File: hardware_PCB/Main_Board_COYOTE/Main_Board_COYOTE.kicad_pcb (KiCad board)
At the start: 2 copper layers, 73.5 x 138 mm, 47 parts, among them J1 FTDI, J2 Conn_01x05_Pin, J3 Conn_01x05_Pin, J4 V+-, J5 MOTOR_PINM1A, J6 MOTOR_PINM1B, J7 MOTOR_PINM1A, J8 MOTOR_PINM1B, Q1 2N7002, SW1 SW_SPST, SW2 START, SW3 START, U1 TA6586, U2 ESP32-WROOM-32, U3 AMS1117-3.3, U4 LM7805_TO220, U5 TA6586

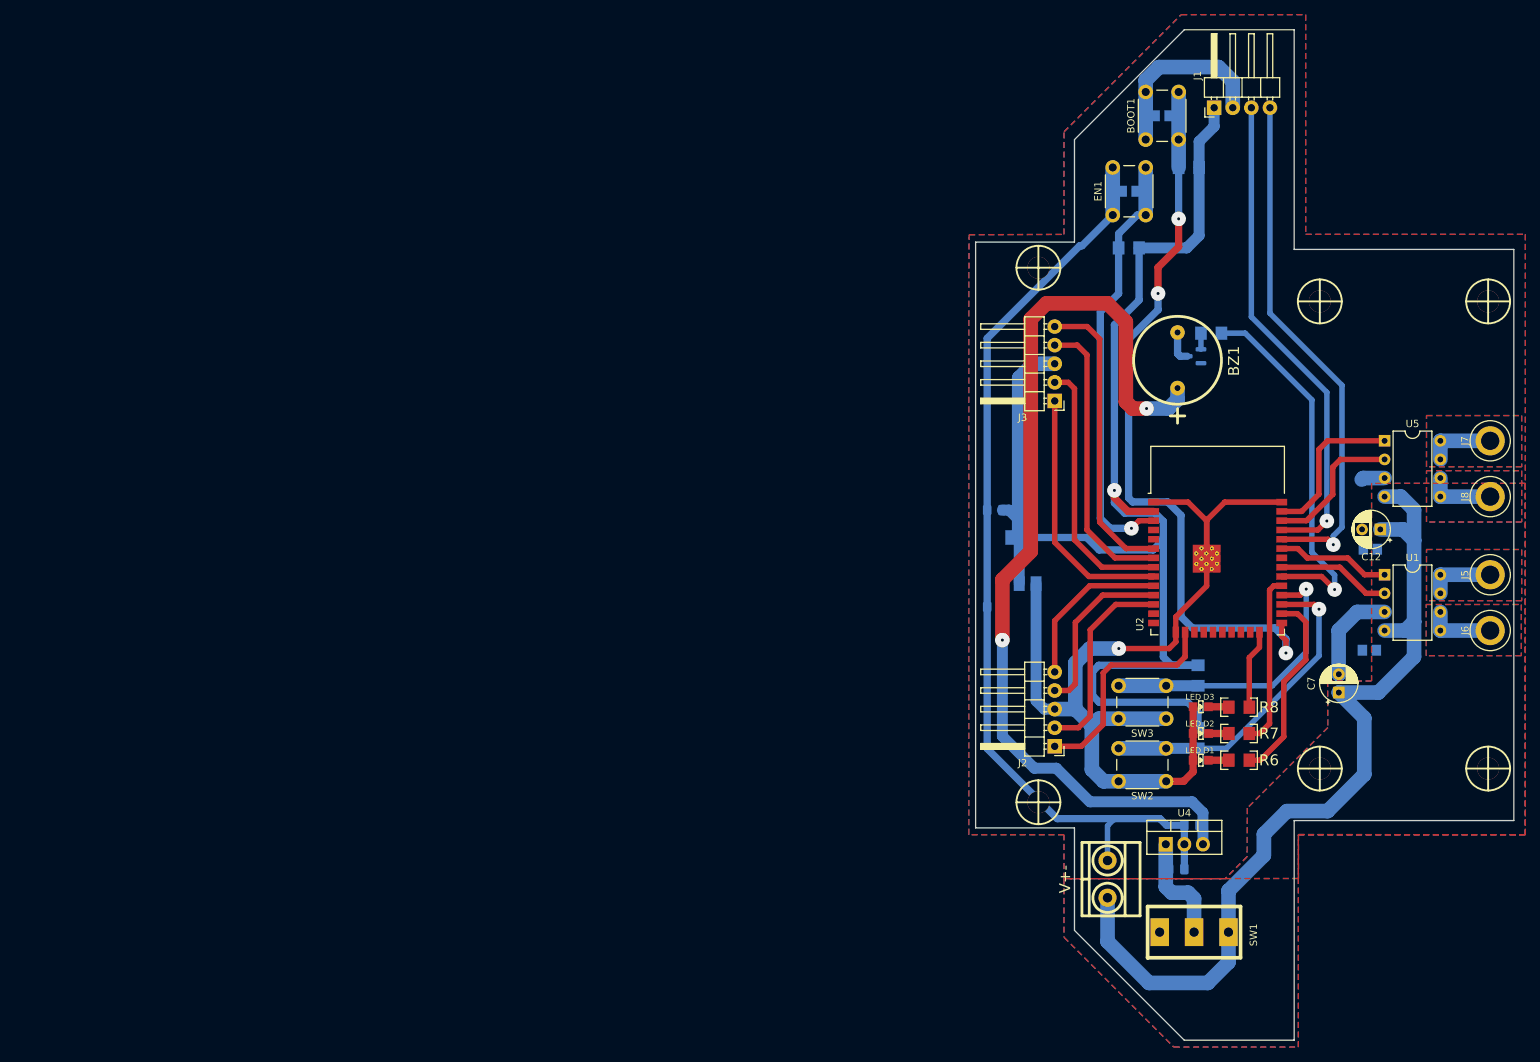
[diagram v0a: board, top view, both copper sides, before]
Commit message: Terminados los PCBs
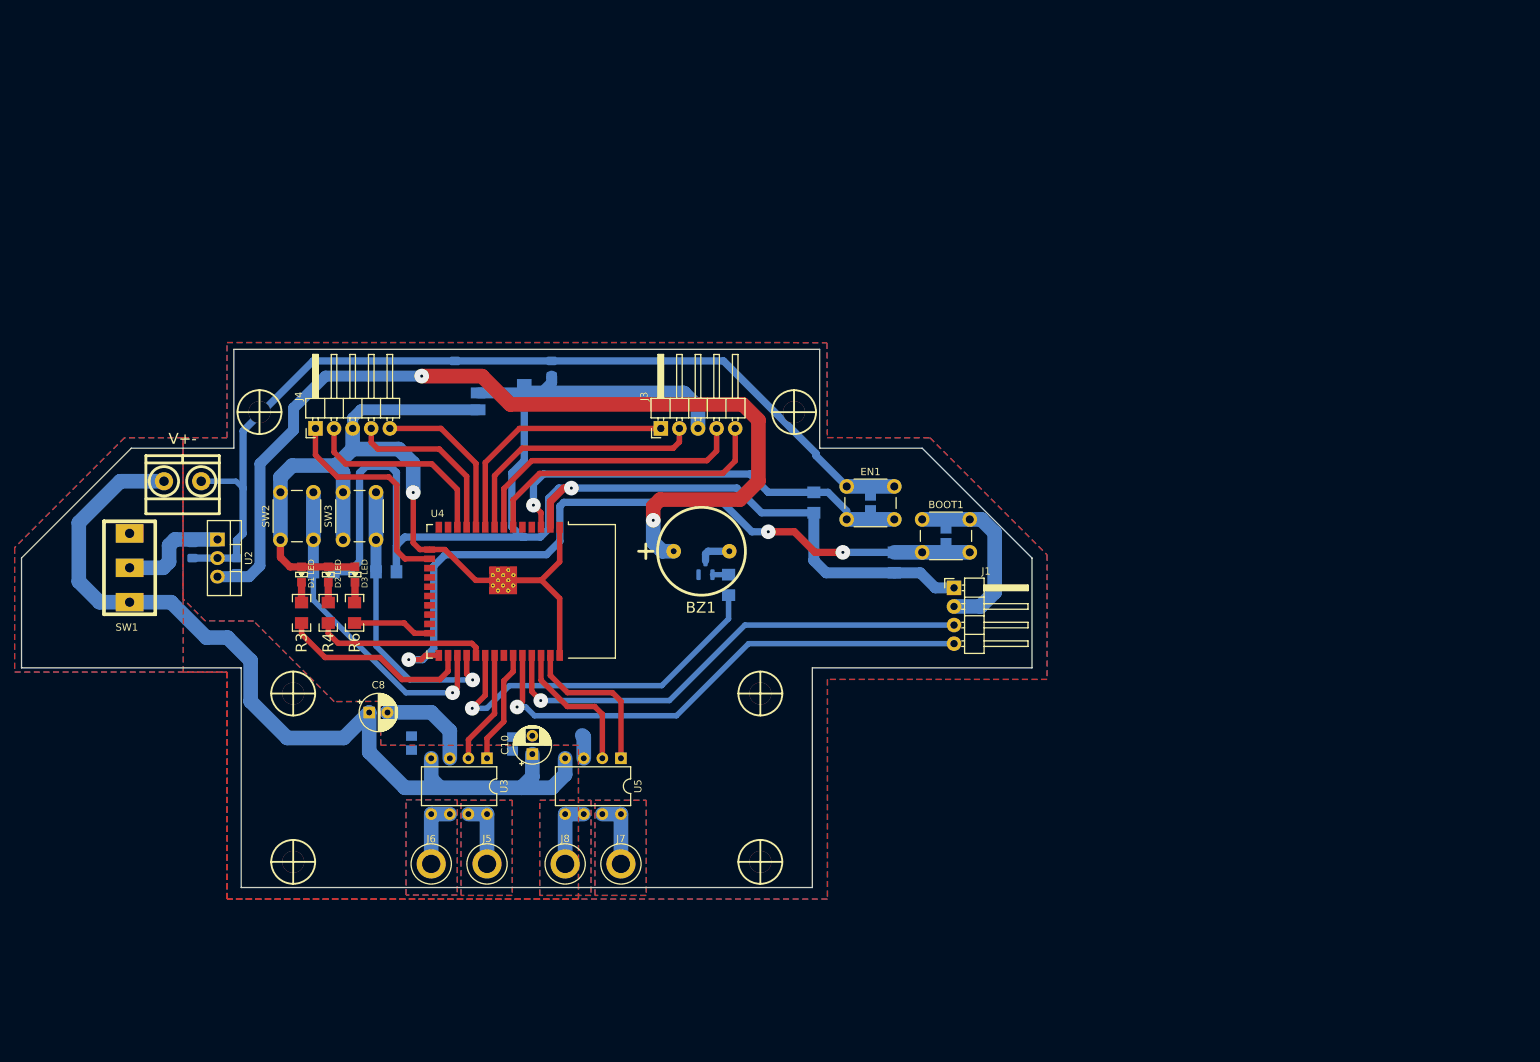
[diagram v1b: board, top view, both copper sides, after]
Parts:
- moved H4 163.7 mm to (96.8, 136.6), turned to -90 degrees
- moved SW1 153.7 mm to (74.5, 96.5), turned to 180 degrees
- moved J6 148.1 mm to (115.7, 136.9), turned to 0 degrees
- moved J5 142.6 mm to (123.3, 136.9), turned to 0 degrees
- moved C2 141.3 mm to (83.1, 94.1), turned to -90 degrees
- moved H1 140.6 mm to (96.8, 113.7), turned to -90 degrees
- moved J2 137.5 mm to (81.7, 84.7), turned to 180 degrees
- moved U2 136.0 mm to (86.5, 92.6), turned to -90 degrees
- moved J8 135.9 mm to (134.0, 136.9), turned to 0 degrees
- moved C5 135.2 mm to (89.1, 96.2), turned to 90 degrees
- moved C8 132.4 mm to (107.2, 116.2), turned to 0 degrees
- moved J7 132.0 mm to (141.6, 136.9), turned to 0 degrees
- moved C9 131.4 mm to (113.0, 120.4), turned to -90 degrees
- moved R3 129.6 mm to (98.0, 102.6), turned to -90 degrees
- moved R4 125.5 mm to (101.6, 102.6), turned to -90 degrees
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- renumbered C8 to C1, C12 to C10, C1 to C2, C5 to C4, C2 to C5, C4 to C6, C6 to C7, C7 to C8, C11 to C9, H2 to H1, H1 to H2, H4 to H3, H3 to H4, J4 to J2, J2 to J4, R2 to R1, R4 to R2, R6 to R3, R7 to R4, R1 to R5, R8 to R6, R3 to R7, R5 to R8, U3 to U1, U4 to U2, U1 to U3, U2 to U4
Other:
- board size 73.5 x 138 mm -> 138 x 73.5 mm
